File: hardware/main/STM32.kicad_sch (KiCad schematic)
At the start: 36 parts, among them U201 REF3430QDGKRQ1, U202 STM32L431RCTx

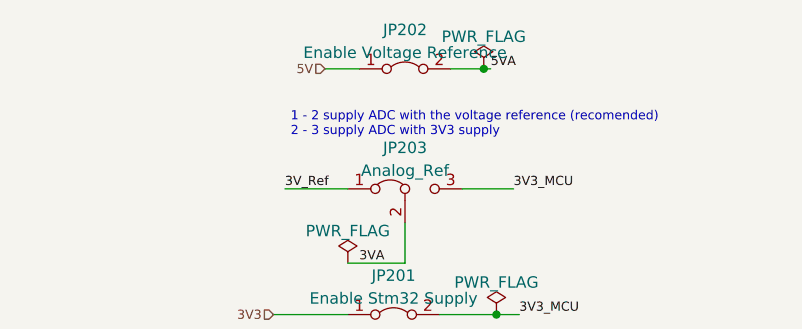
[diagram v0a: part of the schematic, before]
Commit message: Layout: WIP updating control
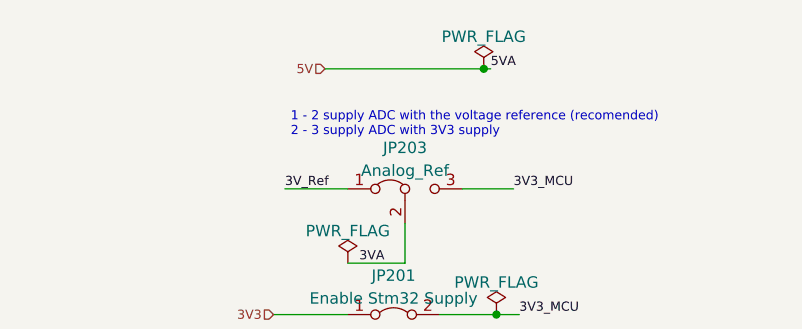
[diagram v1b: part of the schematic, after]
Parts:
- removed JP202: Enable Voltage Reference, Zenite:SolderJumper-2_P0.5mm_Open_TrianglePad0.5x0.5mm, symbol Jumper:Jumper_2_Bridged
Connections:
- net 5VA is gone; now on net 5V: C201.2, C202.2, U201.1 (ENABLE), U201.8 (VIN)
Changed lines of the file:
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@@
-    (stroke (width 0) (type default) (color 0 0 0 0))
-  )
-  (wire (pts (xy 246.38 22.86) (xy 250.053 22.86))
     (stroke (width 0) (type default) (color 0 0 0 0))
   )
@@
     (stroke (width 0) (type default) (color 0 0 0 0))
   )
-  (wire (pts (xy 232.41 22.86) (xy 236.22 22.86))
+  (wire (pts (xy 232.41 22.86) (xy 250.053 22.86))
     (stroke (width 0) (type default) (color 0 0 0 0))
   )
@@
     (pin "1")
   )
-  (symbol (lib_id "Jumper:Jumper_2_Bridged") (at 241.3 22.86 0) (unit 1)
-    (in_bom yes) (on_board yes) (fields_autoplaced)
-    (property "Reference" "JP202" (id 0) (at 241.3 18.5252 0))
-    (property "Value" "Enable Voltage Reference" (id 1) (at 241.3 21.0621 0))
-    (property "Footprint" "Zenite:SolderJumper-2_P0.5mm_Open_TrianglePad0.5x0.5mm" (id 2) (at 241.3 22.86 0)
-      (effects (font (size 1.27 1.27)) hide)
-    )
-    (property "Datasheet" "~" (id 3) (at 241.3 22.86 0)
-      (effects (font (size 1.27 1.27)) hide)
-    )
-    (pin "1")
-    (pin "2")
-  )
   (symbol (lib_id "Jumper:Jumper_2_Bridged") (at 240.03 50.165 0) (unit 1)
